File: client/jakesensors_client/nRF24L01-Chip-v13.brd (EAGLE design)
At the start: 16 x 32.6 mm, 26 parts, among them IC1 BME280, Q1 16MHz, U1 NRF24, U4 RPI-103X, Y1 ANTENNA2SMD5

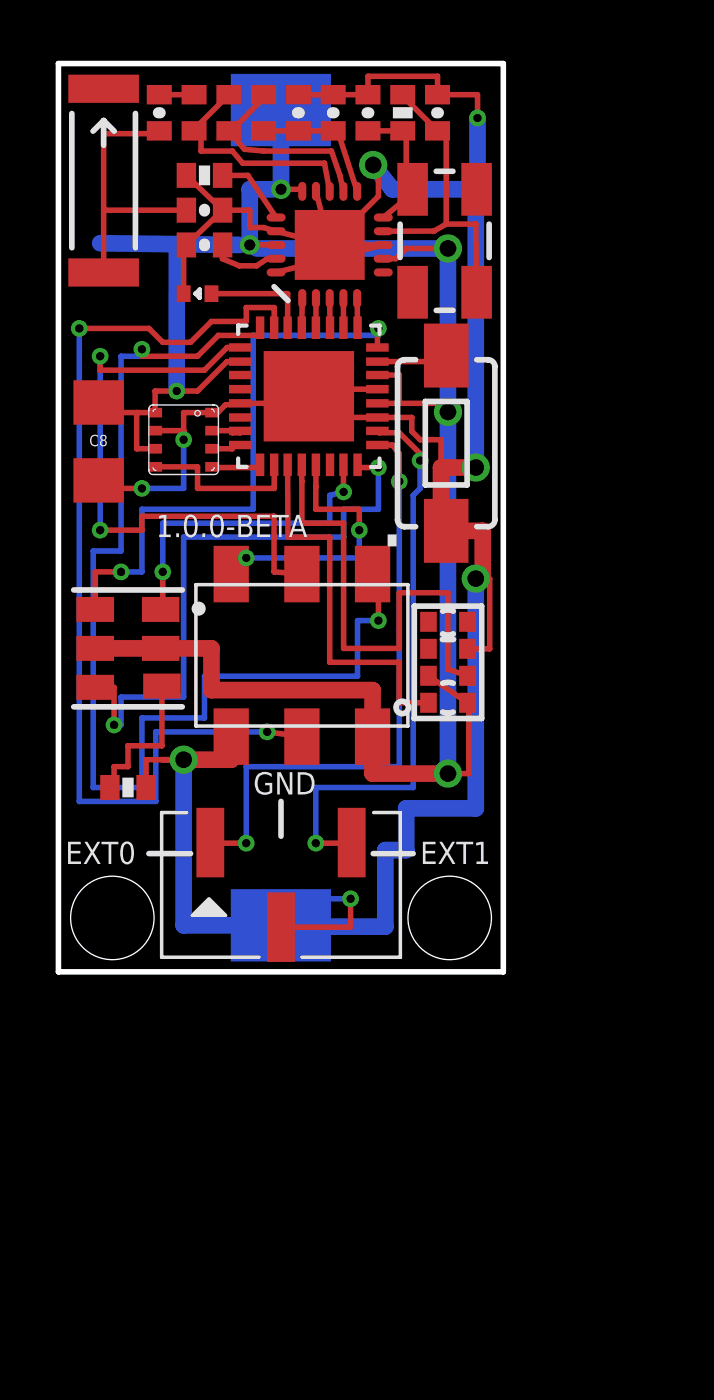
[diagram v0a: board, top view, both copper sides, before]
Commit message: start of server
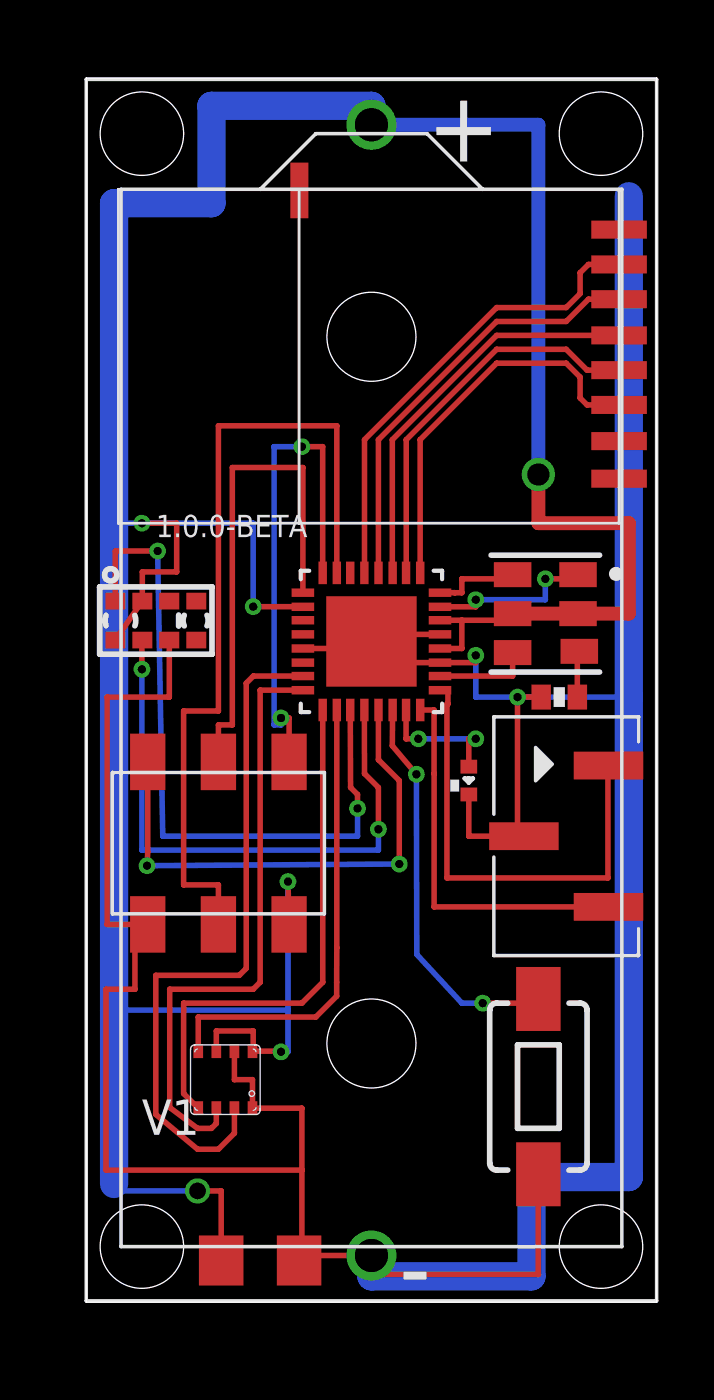
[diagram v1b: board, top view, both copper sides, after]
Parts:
- removed BT1: CR2032-HOLDER, battery-holder:CH28-2032LF
- removed C1, C2: 22pF, SparkFun:0402-CAP
- removed C3: 33nF, SparkFun:0402-CAP
- removed C4: 2.2nF, SparkFun:0402-CAP
- removed C5: 4.7pF, SparkFun:0402-CAP
- removed C6: 1.0pF, SparkFun:0402-CAP
- removed C7: 1.5pF, SparkFun:0402-CAP
- removed L1: 3.9nH, SparkFun:C0402
- removed L2: 2.7nH, SparkFun:C0402
- removed L3: 8.2nH, SparkFun:C0402
- removed Q1: 16MHz, SparkFun:CRYSTAL-SMD-5X3
- removed R1: 1M, SparkFun:0402-RES
- removed R2: 22K, SparkFun:0402-RES
- removed U1: NRF24, Testing:QFN20_ALT1
- removed Y1: ANTENNA2SMD5, SparkFun:ANTENNA-CHIP5
- added U$1: NRF24L01+, NRF:NRF24L01+
- added V1: (no value), battery_xtra:TAKACHI_CR123A
- moved C8 30.0 mm to (31.5, 9.50), turned to 0 degrees
- moved S1 23.4 mm to (41.5, 15.8)
- moved IC1 23.0 mm to (30.2, 16.0), turned to 0 degrees
- moved LED1 20.0 mm to (39.0, 26.8), turned to 90 degrees
- moved R3 15.8 mm to (42.2, 29.8), turned to 180 degrees
- moved U4 15.1 mm to (41.8, 32.8)
- moved U3 10.6 mm to (27.8, 32.5), turned to 90 degrees
- moved JP1 10.4 mm to (42.5, 24.8), turned to 270 degrees
- moved U2 9.10 mm to (35.5, 31.8)
- moved P1 7.39 mm to (30.0, 24.5)
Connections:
- removed net ANT: C6.2, C7.2, Y1.FEED
- removed net N$22: U1.2, U2.12
- removed net N$26: LED1.A, U2.14
- removed net N$3 (its old number): L2.2, L3.1, U1.12
- removed net N$4: R2.1, U1.16
- removed net N$5: C3.1, U1.19
- removed net N$6: L1.1, L3.2, U1.13
- removed net N$7: C4.1, C5.1, L2.1, U1.11
- removed net N$9: C7.1, L1.2
- net GND: now also V1.-; no longer BT1.NEG, C1.2, C2.2, C3.2, C4.2, C5.2, C6.1, R2.2, U1.0, U1.14, U1.17, U1.20, U1.8
- net N$1: now also U$1.6, U2.12; no longer C1.1, Q1.1, R1.1, U1.9
- net N$18: now also U$1.3; no longer U1.5
- net N$19: now also U$1.4; no longer U1.4
- net N$2: now also LED1.A, U2.31; no longer C2.1, Q1.3, R1.2, U1.10
- net N$21: now also U$1.5; no longer U1.3
- net N$24: now also U2.32; no longer U2.2
- net N$28: now also U2.30; no longer U2.7
- net N$29: now also U2.2; no longer U2.32
- net N$30: now also U2.7; no longer U2.31
- net N$37: now also U$1.7; no longer U1.1
- net VCC: now also V1.+; no longer BT1.POS, U1.15, U1.18, U1.7
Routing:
- net VCC: track 82.2 -> 125.7 mm
- net N$23: track 1.15 -> 25.2 mm
- net N$13: track 40.8 -> 18.7 mm
- net N$3: track 1.15 -> 22.2 mm
- net N$29: track 21.6 -> 3.46 mm, vias 2 -> 0
- net N$31: track 21.0 -> 3.18 mm, vias 2 -> 0
- net N$17: track 2.32 -> 19.1 mm
- net N$37: track 1.05 -> 17.0 mm
- net N$21: track 1.05 -> 14.5 mm
- net N$18: track 1.05 -> 14.1 mm
- net N$19: track 1.05 -> 14.1 mm
- net N$28: track 2.56 -> 14.3 mm, vias 0 -> 2
- net N$15: track 13.6 -> 25.2 mm, vias 0 -> 2
- net N$8: track 5.90 -> 16.8 mm
- net ANT: track 10.5 -> 0.00 mm
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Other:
- board size 16 x 32.6 mm -> 20.5 x 44 mm
- board text removed: "EXT0"
- board text removed: "EXT1"
- board text removed: "GND"
